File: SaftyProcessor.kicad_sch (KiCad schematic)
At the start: 48 parts, among them J1 1935161, J2 1935161, J3 SJ2-35813B-SMT-TR, J4 SJ2-35813B-SMT-TR, J5 1935161, U1 LM7805_TO220, U2 LM1117T-3.3, U4 TCMT1109, U5 TCMT1109, U6 TCMT1109

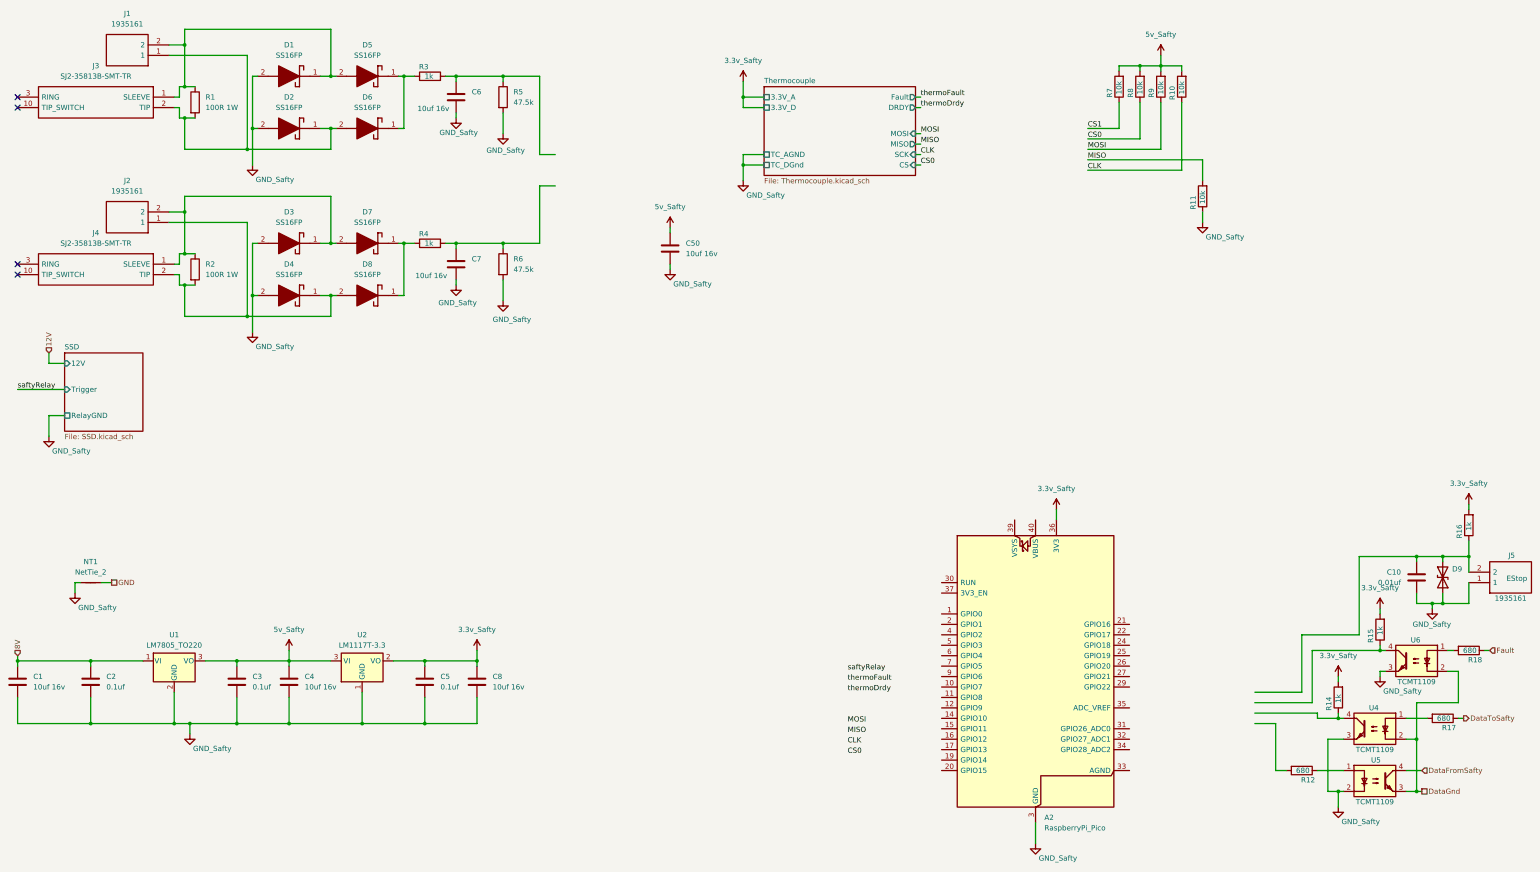
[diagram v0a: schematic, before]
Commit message: sch progress
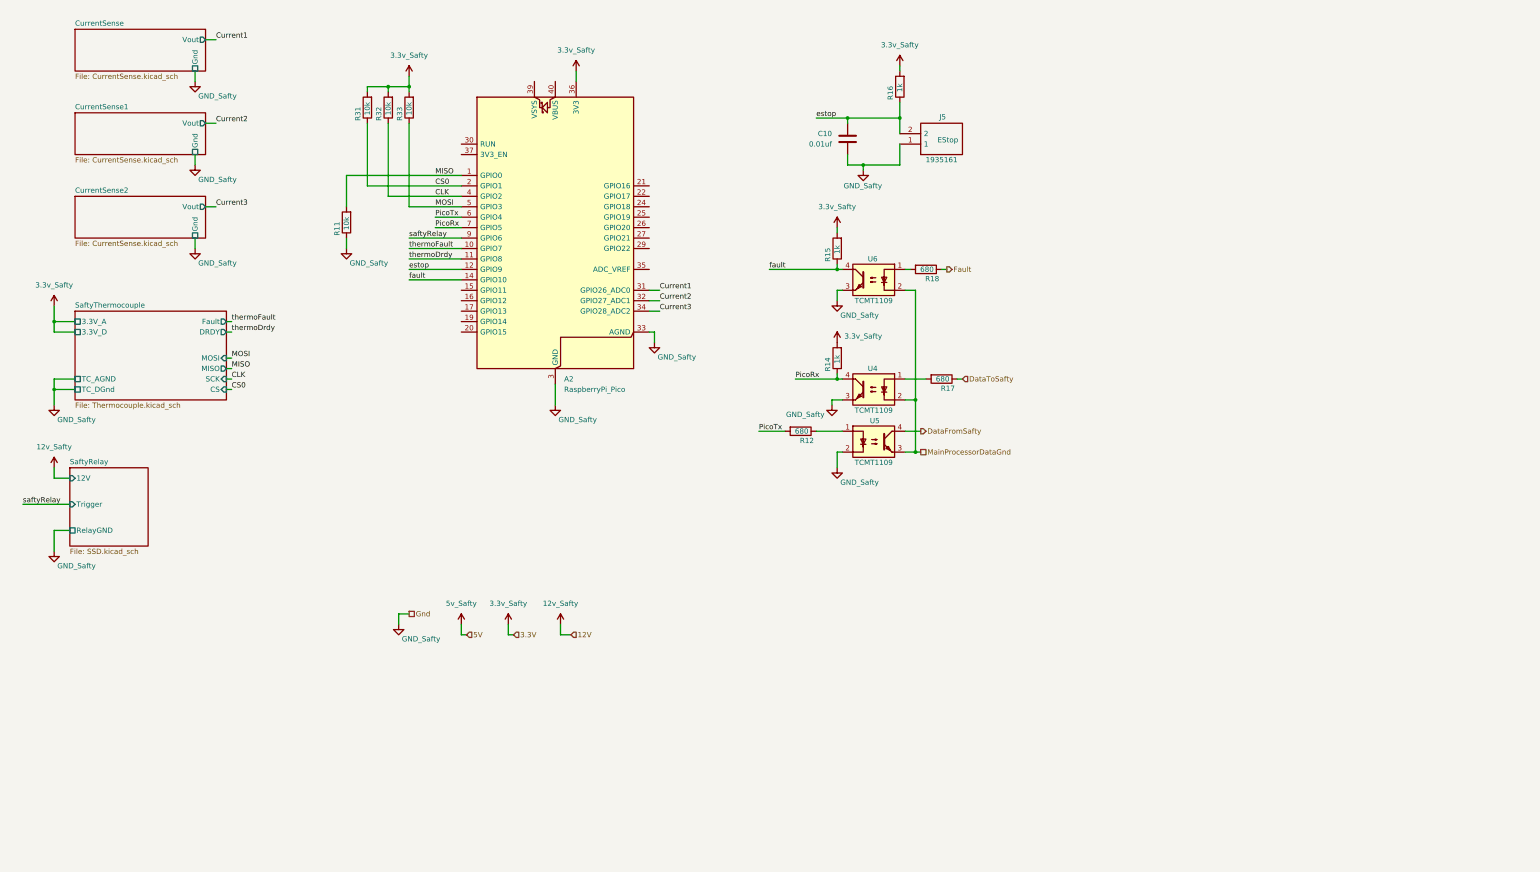
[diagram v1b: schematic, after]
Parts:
- removed C1, C4, C50, C6, C7, C8: 10uf 16v, Capacitor_SMD:C_0805_2012Metric, symbol Device:C
- removed C2, C3, C5: 0.1uf, Capacitor_SMD:C_0402_1005Metric, symbol Device:C
- removed D1, D2, D3, D4, D5, D6, D7, D8: SS16FP, SamacSys_Parts:SS12FP, symbol SamacSys_Parts:SS16FP
- removed D9: SMAJ24CA, Diode_SMD:D_SMA, symbol Diode:SMAJ24CA
- removed J1, J2: 1935161, SamacSys_Parts:1935161, symbol SamacSys_Parts:1935161
- removed J3, J4: SJ2-35813B-SMT-TR, SamacSys_Parts:SJ235813BSMTTR, symbol SamacSys_Parts:SJ2-35813B-SMT-TR
- removed NT1: NetTie_2, symbol Device:NetTie_2
- removed R1, R2: 100R 1W, Resistor_SMD:R_2512_6332Metric, symbol Device:R
- removed R10, R7, R8, R9: 10k, Resistor_SMD:R_0402_1005Metric, symbol Device:R
- removed R3, R4: 1k, Resistor_SMD:R_0402_1005Metric, symbol Device:R
- removed R5, R6: 47.5k, Resistor_SMD:R_0402_1005Metric, symbol Device:R
- removed U1: LM7805_TO220, Package_TO_SOT_THT:TO-220-3_Vertical, symbol Regulator_Linear:LM7805_TO220
- removed U2: LM1117T-3.3, Package_TO_SOT_THT:TO-220-3_Vertical, symbol Regulator_Linear:LM1117T-3.3
- added R31, R32, R33: 10k, Resistor_SMD:R_0402_1005Metric, symbol Device:R
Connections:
- net 3.3v_Safty: now also R31.2, R32.2, R33.2
- net CLK: now also A2.4 (GPIO2), R32.1
- net CS0: now also A2.2 (GPIO1), R31.1
- net GND_Safty: now also A2.33 (AGND)
- net MISO: now also A2.1 (GPIO0)
- net MOSI: now also A2.5 (GPIO3), R33.1
- net saftyRelay: now also A2.9 (GPIO6)
- net thermoDrdy: now also A2.11 (GPIO8)
- net thermoFault: now also A2.10 (GPIO7)
- net PicoTx: now reaches R12.2
- net PicoTx: now also A2.6 (GPIO4)
- net estop: now reaches C10.1, J5.2, R16.1
- net estop: now also A2.12 (GPIO9)
- net fault: now reaches R15.1, U6.4
- net fault: now also A2.14 (GPIO10)
- net PicoRx: now reaches R14.1, U4.4
- net PicoRx: now also A2.7 (GPIO5)
- net Current1: now reaches A2.31 (GPIO26_ADC0)
- net Current2: now reaches A2.32 (GPIO27_ADC1)
- net Current3: now reaches A2.34 (GPIO28_ADC2)
- net DataGnd renamed MainProcessorDataGnd
- no-connect marks 4 -> 0
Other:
- sheet SSD renamed SaftyRelay
- removed sheet Thermocouple
- added sheet CurrentSense (CurrentSense.kicad_sch)
- added sheet CurrentSense1 (CurrentSense.kicad_sch)
- added sheet CurrentSense2 (CurrentSense.kicad_sch)
- added sheet SaftyThermocouple (Thermocouple.kicad_sch)
- moved on the sheet: A2, C10, J5, R12, R14, R15, R16, R17, R18, U4, U5, U6
